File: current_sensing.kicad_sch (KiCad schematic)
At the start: 6 parts, among them U10 INA181A1

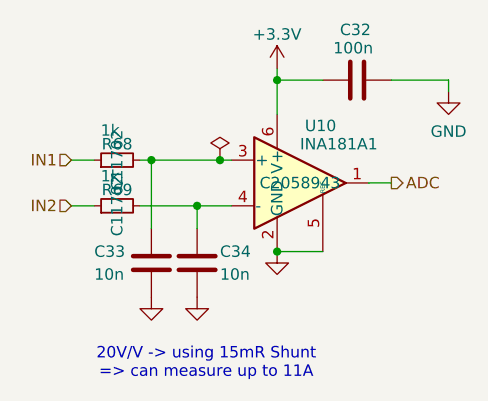
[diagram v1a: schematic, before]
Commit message: started silkscrean
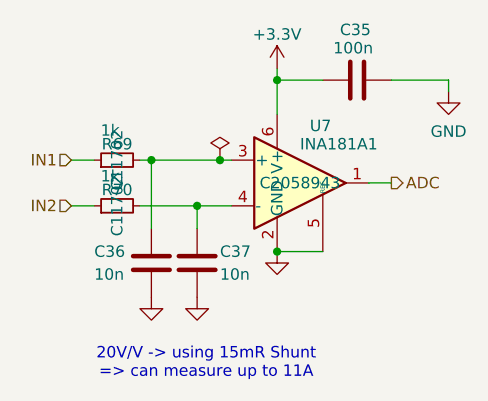
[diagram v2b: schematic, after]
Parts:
- renumbered C32 to C35, C33 to C36, C34 to C37, R68 to R69, R69 to R70, U10 to U7
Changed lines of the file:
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@@
 		(on_board yes)
 		(dnp no)
-		(property "Reference" "U10"
+		(property "Reference" "U7"
 			(at 124.206 82.55 0)
 			(effects
@@
 			(project "frodo_io_module"
 				(path "/c1ccca3c-4648-4b8e-86a1-690c24c5f13e/0381ad7c-a4fe-46cf-80e9-20458dbb02ae"
-					(reference "U11")
-					(unit 1)
-				)
-				(path "/c1ccca3c-4648-4b8e-86a1-690c24c5f13e/503665e4-7dbc-4cb7-9fc2-35263499a935"
-					(reference "U1")
-					(unit 1)
-				)
-				(path "/c1ccca3c-4648-4b8e-86a1-690c24c5f13e/b9f805af-f42c-49d8-9c2b-cbc55b6b7bfe"
-					(reference "U10")
+					(reference "U8")
+					(unit 1)
+				)
+				(path "/c1ccca3c-4648-4b8e-86a1-690c24c5f13e/503665e4-7dbc-4cb7-9fc2-35263499a935"
+					(reference "U9")
+					(unit 1)
+				)
+				(path "/c1ccca3c-4648-4b8e-86a1-690c24c5f13e/b9f805af-f42c-49d8-9c2b-cbc55b6b7bfe"
+					(reference "U7")
 					(unit 1)
 				)
@@
 		(on_board yes)
 		(dnp no)
-		(property "Reference" "C32"
+		(property "Reference" "C35"
 			(at 129.794 71.882 90)
 			(effects
@@
 			(project "frodo_io_module"
 				(path "/c1ccca3c-4648-4b8e-86a1-690c24c5f13e/0381ad7c-a4fe-46cf-80e9-20458dbb02ae"
+					(reference "C38")
+					(unit 1)
+				)
+				(path "/c1ccca3c-4648-4b8e-86a1-690c24c5f13e/503665e4-7dbc-4cb7-9fc2-35263499a935"
+					(reference "C41")
+					(unit 1)
+				)
+				(path "/c1ccca3c-4648-4b8e-86a1-690c24c5f13e/b9f805af-f42c-49d8-9c2b-cbc55b6b7bfe"
 					(reference "C35")
-					(unit 1)
-				)
-				(path "/c1ccca3c-4648-4b8e-86a1-690c24c5f13e/503665e4-7dbc-4cb7-9fc2-35263499a935"
-					(reference "C38")
-					(unit 1)
-				)
-				(path "/c1ccca3c-4648-4b8e-86a1-690c24c5f13e/b9f805af-f42c-49d8-9c2b-cbc55b6b7bfe"
-					(reference "C32")
 					(unit 1)
 				)
@@
 		(on_board yes)
 		(dnp no)
-		(property "Reference" "R69"
+		(property "Reference" "R70"
 			(at 101.6 89.662 90)
 			(effects
@@
 			(project "frodo_io_module"
 				(path "/c1ccca3c-4648-4b8e-86a1-690c24c5f13e/0381ad7c-a4fe-46cf-80e9-20458dbb02ae"
-					(reference "R71")
-					(unit 1)
-				)
-				(path "/c1ccca3c-4648-4b8e-86a1-690c24c5f13e/503665e4-7dbc-4cb7-9fc2-35263499a935"
-					(reference "R16")
-					(unit 1)
-				)
-				(path "/c1ccca3c-4648-4b8e-86a1-690c24c5f13e/b9f805af-f42c-49d8-9c2b-cbc55b6b7bfe"
-					(reference "R69")
+					(reference "R72")
+					(unit 1)
+				)
+				(path "/c1ccca3c-4648-4b8e-86a1-690c24c5f13e/503665e4-7dbc-4cb7-9fc2-35263499a935"
+					(reference "R74")
+					(unit 1)
+				)
+				(path "/c1ccca3c-4648-4b8e-86a1-690c24c5f13e/b9f805af-f42c-49d8-9c2b-cbc55b6b7bfe"
+					(reference "R70")
 					(unit 1)
 				)
@@
 				)
 				(path "/c1ccca3c-4648-4b8e-86a1-690c24c5f13e/503665e4-7dbc-4cb7-9fc2-35263499a935"
-					(reference "#FLG05")
+					(reference "#FLG010")
 					(unit 1)
 				)
@@
 		(dnp no)
 		(fields_autoplaced yes)
-		(property "Reference" "#PWR0135"
+		(property "Reference" "#PWR0122"
 			(at 138.43 85.09 0)
 			(effects
@@
 			(project "frodo_io_module"
 				(path "/c1ccca3c-4648-4b8e-86a1-690c24c5f13e/0381ad7c-a4fe-46cf-80e9-20458dbb02ae"
-					(reference "#PWR0140")
-					(unit 1)
-				)
-				(path "/c1ccca3c-4648-4b8e-86a1-690c24c5f13e/503665e4-7dbc-4cb7-9fc2-35263499a935"
-					(reference "#PWR017")
-					(unit 1)
-				)
-				(path "/c1ccca3c-4648-4b8e-86a1-690c24c5f13e/b9f805af-f42c-49d8-9c2b-cbc55b6b7bfe"
-					(reference "#PWR0135")
+					(reference "#PWR0127")
+					(unit 1)
+				)
+				(path "/c1ccca3c-4648-4b8e-86a1-690c24c5f13e/503665e4-7dbc-4cb7-9fc2-35263499a935"
+					(reference "#PWR0132")
+					(unit 1)
+				)
+				(path "/c1ccca3c-4648-4b8e-86a1-690c24c5f13e/b9f805af-f42c-49d8-9c2b-cbc55b6b7bfe"
+					(reference "#PWR0122")
 					(unit 1)
 				)
@@
 		(on_board yes)
 		(dnp no)
-		(property "Reference" "#PWR0134"
+		(property "Reference" "#PWR0121"
 			(at 119.38 80.01 0)
 			(effects
@@
 			(project "frodo_io_module"
 				(path "/c1ccca3c-4648-4b8e-86a1-690c24c5f13e/0381ad7c-a4fe-46cf-80e9-20458dbb02ae"
-					(reference "#PWR0139")
-					(unit 1)
-				)
-				(path "/c1ccca3c-4648-4b8e-86a1-690c24c5f13e/503665e4-7dbc-4cb7-9fc2-35263499a935"
-					(reference "#PWR016")
-					(unit 1)
-				)
-				(path "/c1ccca3c-4648-4b8e-86a1-690c24c5f13e/b9f805af-f42c-49d8-9c2b-cbc55b6b7bfe"
-					(reference "#PWR0134")
+					(reference "#PWR0126")
+					(unit 1)
+				)
+				(path "/c1ccca3c-4648-4b8e-86a1-690c24c5f13e/503665e4-7dbc-4cb7-9fc2-35263499a935"
+					(reference "#PWR0131")
+					(unit 1)
+				)
+				(path "/c1ccca3c-4648-4b8e-86a1-690c24c5f13e/b9f805af-f42c-49d8-9c2b-cbc55b6b7bfe"
+					(reference "#PWR0121")
 					(unit 1)
 				)
@@
 		(on_board yes)
 		(dnp no)
-		(property "Reference" "R68"
+		(property "Reference" "R69"
 			(at 101.6 84.582 90)
 			(effects
@@
 			(project "frodo_io_module"
 				(path "/c1ccca3c-4648-4b8e-86a1-690c24c5f13e/0381ad7c-a4fe-46cf-80e9-20458dbb02ae"
-					(reference "R70")
-					(unit 1)
-				)
-				(path "/c1ccca3c-4648-4b8e-86a1-690c24c5f13e/503665e4-7dbc-4cb7-9fc2-35263499a935"
-					(reference "R15")
-					(unit 1)
-				)
-				(path "/c1ccca3c-4648-4b8e-86a1-690c24c5f13e/b9f805af-f42c-49d8-9c2b-cbc55b6b7bfe"
-					(reference "R68")
+					(reference "R71")
+					(unit 1)
+				)
+				(path "/c1ccca3c-4648-4b8e-86a1-690c24c5f13e/503665e4-7dbc-4cb7-9fc2-35263499a935"
+					(reference "R73")
+					(unit 1)
+				)
+				(path "/c1ccca3c-4648-4b8e-86a1-690c24c5f13e/b9f805af-f42c-49d8-9c2b-cbc55b6b7bfe"
+					(reference "R69")
 					(unit 1)
 				)
@@
 		(on_board yes)
 		(dnp no)
-		(property "Reference" "C33"
+		(property "Reference" "C36"
 			(at 99.06 96.52 0)
 			(effects
@@
 			(project "frodo_io_module"
 				(path "/c1ccca3c-4648-4b8e-86a1-690c24c5f13e/0381ad7c-a4fe-46cf-80e9-20458dbb02ae"
+					(reference "C39")
+					(unit 1)
+				)
+				(path "/c1ccca3c-4648-4b8e-86a1-690c24c5f13e/503665e4-7dbc-4cb7-9fc2-35263499a935"
+					(reference "C42")
+					(unit 1)
+				)
+				(path "/c1ccca3c-4648-4b8e-86a1-690c24c5f13e/b9f805af-f42c-49d8-9c2b-cbc55b6b7bfe"
 					(reference "C36")
-					(unit 1)
-				)
-				(path "/c1ccca3c-4648-4b8e-86a1-690c24c5f13e/503665e4-7dbc-4cb7-9fc2-35263499a935"
-					(reference "C40")
-					(unit 1)
-				)
-				(path "/c1ccca3c-4648-4b8e-86a1-690c24c5f13e/b9f805af-f42c-49d8-9c2b-cbc55b6b7bfe"
-					(reference "C33")
 					(unit 1)
 				)
@@
 		(on_board yes)
 		(dnp no)
-		(property "Reference" "C34"
+		(property "Reference" "C37"
 			(at 113.03 96.52 0)
 			(effects
@@
 			(project "frodo_io_module"
 				(path "/c1ccca3c-4648-4b8e-86a1-690c24c5f13e/0381ad7c-a4fe-46cf-80e9-20458dbb02ae"
+					(reference "C40")
+					(unit 1)
+				)
+				(path "/c1ccca3c-4648-4b8e-86a1-690c24c5f13e/503665e4-7dbc-4cb7-9fc2-35263499a935"
+					(reference "C43")
+					(unit 1)
+				)
+				(path "/c1ccca3c-4648-4b8e-86a1-690c24c5f13e/b9f805af-f42c-49d8-9c2b-cbc55b6b7bfe"
 					(reference "C37")
-					(unit 1)
-				)
-				(path "/c1ccca3c-4648-4b8e-86a1-690c24c5f13e/503665e4-7dbc-4cb7-9fc2-35263499a935"
-					(reference "C41")
-					(unit 1)
-				)
-				(path "/c1ccca3c-4648-4b8e-86a1-690c24c5f13e/b9f805af-f42c-49d8-9c2b-cbc55b6b7bfe"
-					(reference "C34")
 					(unit 1)
 				)
@@
 		(dnp no)
 		(fields_autoplaced yes)
-		(property "Reference" "#PWR0136"
+		(property "Reference" "#PWR0123"
 			(at 119.38 102.87 0)
 			(effects
@@
 			(project "frodo_io_module"
 				(path "/c1ccca3c-4648-4b8e-86a1-690c24c5f13e/0381ad7c-a4fe-46cf-80e9-20458dbb02ae"
-					(reference "#PWR0141")
-					(unit 1)
-				)
-				(path "/c1ccca3c-4648-4b8e-86a1-690c24c5f13e/503665e4-7dbc-4cb7-9fc2-35263499a935"
-					(reference "#PWR019")
-					(unit 1)
-				)
-				(path "/c1ccca3c-4648-4b8e-86a1-690c24c5f13e/b9f805af-f42c-49d8-9c2b-cbc55b6b7bfe"
-					(reference "#PWR0136")
+					(reference "#PWR0128")
+					(unit 1)
+				)
+				(path "/c1ccca3c-4648-4b8e-86a1-690c24c5f13e/503665e4-7dbc-4cb7-9fc2-35263499a935"
+					(reference "#PWR0133")
+					(unit 1)
+				)
+				(path "/c1ccca3c-4648-4b8e-86a1-690c24c5f13e/b9f805af-f42c-49d8-9c2b-cbc55b6b7bfe"
+					(reference "#PWR0123")
 					(unit 1)
 				)
@@
 		(dnp no)
 		(fields_autoplaced yes)
-		(property "Reference" "#PWR0138"
+		(property "Reference" "#PWR0125"
 			(at 110.49 107.95 0)
 			(effects
@@
 			(project "frodo_io_module"
 				(path "/c1ccca3c-4648-4b8e-86a1-690c24c5f13e/0381ad7c-a4fe-46cf-80e9-20458dbb02ae"
-					(reference "#PWR0143")
-					(unit 1)
-				)
-				(path "/c1ccca3c-4648-4b8e-86a1-690c24c5f13e/503665e4-7dbc-4cb7-9fc2-35263499a935"
-					(reference "#PWR034")
-					(unit 1)
-				)
-				(path "/c1ccca3c-4648-4b8e-86a1-690c24c5f13e/b9f805af-f42c-49d8-9c2b-cbc55b6b7bfe"
-					(reference "#PWR0138")
+					(reference "#PWR0130")
+					(unit 1)
+				)
+				(path "/c1ccca3c-4648-4b8e-86a1-690c24c5f13e/503665e4-7dbc-4cb7-9fc2-35263499a935"
+					(reference "#PWR0135")
+					(unit 1)
+				)
+				(path "/c1ccca3c-4648-4b8e-86a1-690c24c5f13e/b9f805af-f42c-49d8-9c2b-cbc55b6b7bfe"
+					(reference "#PWR0125")
 					(unit 1)
 				)
@@
 		(dnp no)
 		(fields_autoplaced yes)
-		(property "Reference" "#PWR0137"
+		(property "Reference" "#PWR0124"
 			(at 105.41 107.95 0)
 			(effects
@@
 			(project "frodo_io_module"
 				(path "/c1ccca3c-4648-4b8e-86a1-690c24c5f13e/0381ad7c-a4fe-46cf-80e9-20458dbb02ae"
-					(reference "#PWR0142")
-					(unit 1)
-				)
-				(path "/c1ccca3c-4648-4b8e-86a1-690c24c5f13e/503665e4-7dbc-4cb7-9fc2-35263499a935"
-					(reference "#PWR023")
-					(unit 1)
-				)
-				(path "/c1ccca3c-4648-4b8e-86a1-690c24c5f13e/b9f805af-f42c-49d8-9c2b-cbc55b6b7bfe"
-					(reference "#PWR0137")
-					(unit 1)
-				)
+					(reference "#PWR0129")
+					(unit 1)
+				)
+				(path "/c1ccca3c-4648-4b8e-86a1-690c24c5f13e/503665e4-7dbc-4cb7-9fc2-35263499a935"
+					(reference "#PWR0134")
+					(unit 1)
+				)
+				(path "/c1ccca3c-4648-4b8e-86a1-690c24c5f13e/b9f805af-f42c-49d8-9c2b-cbc55b6b7bfe"
+					(reference "#PWR0124")
+					(unit 1)
+				)
